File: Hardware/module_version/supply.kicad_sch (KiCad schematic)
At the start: 21 parts, among them J21 Power Input, U32 TLV1117LV33DCYR, U33 TX4139

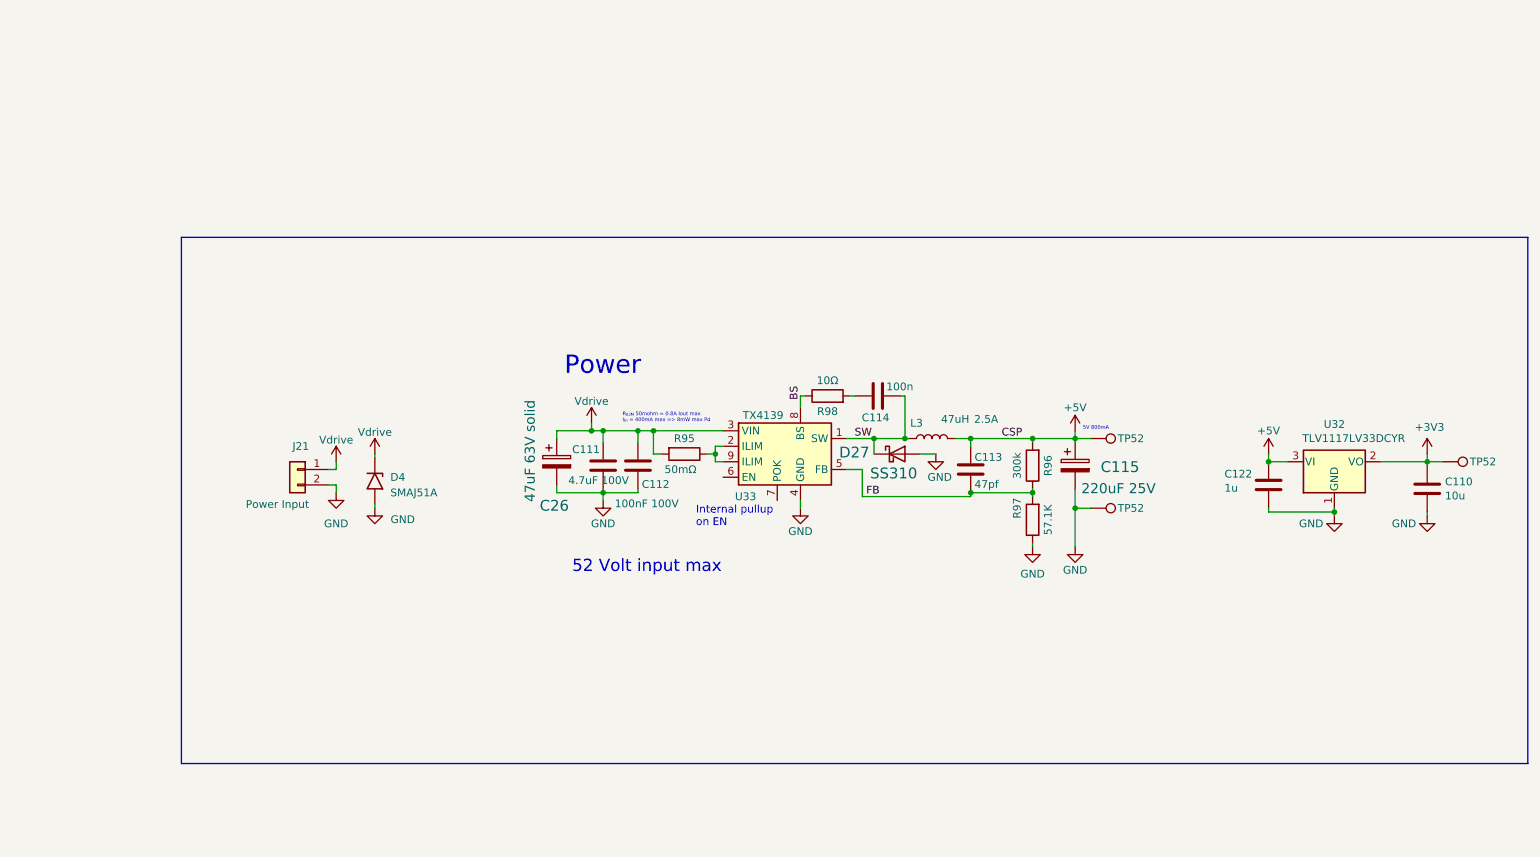
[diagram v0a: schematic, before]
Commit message: work in progress...
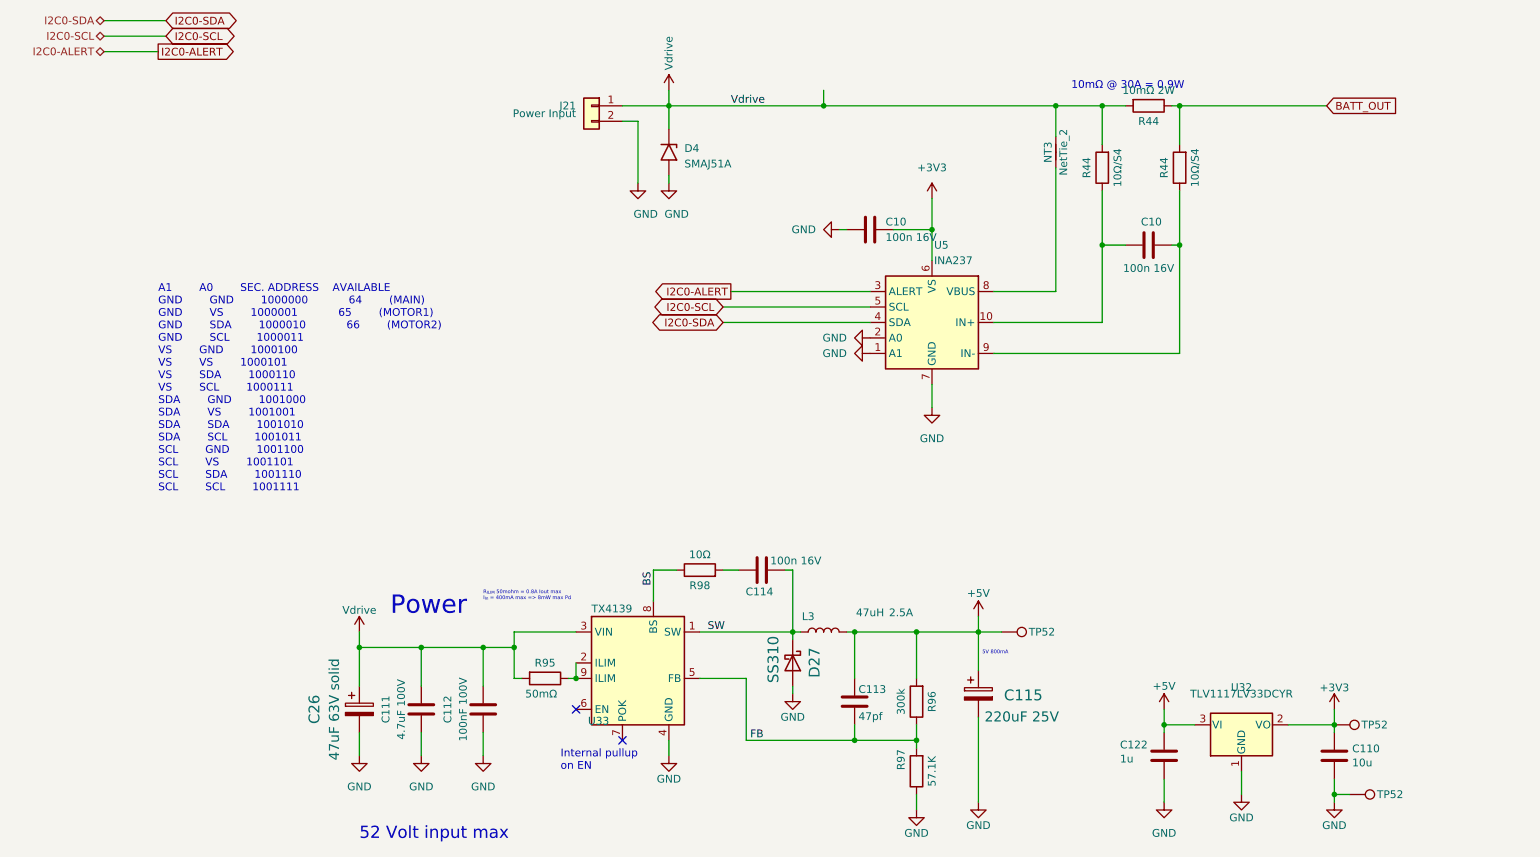
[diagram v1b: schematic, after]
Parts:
- added C10 (x2): 100n 16V, Capacitor_SMD:C_0402_1005Metric, symbol Device:C
- added NT3: NetTie_2, NetTie:NetTie-2_SMD_Pad0.5mm, symbol Device:NetTie_2
- added R44: 10mΩ 2W, Resistor_SMD:R_2512_6332Metric_Pad1.40x3.35mm_HandSolder, symbol Device:R
- added R44 (x2): 10Ω/S4, Resistor_SMD:R_0402_1005Metric, symbol Device:R
- added U5: INA237, Package_SO:VSSOP-10_3x3mm_P0.5mm, symbol katodo_kicad:INA237
- C114: value 100n -> 100n 16V; footprint Capacitor_SMD:C_0603_1608Metric -> Capacitor_SMD:C_0402_1005Metric; LCSC C14663 -> C60474; MFR (none) -> CC0402KRX7R7BB104
- R98: footprint Resistor_SMD:R_0603_1608Metric -> Resistor_SMD:R_0402_1005Metric_Pad0.72x0.64mm_HandSolder; LCSC C22859 -> C138066
- U32: symbol Regulator_Linear:NCP1117-3.3_SOT223 -> katodo_kicad:NCP1117-3.3_SOT223
- U33: symbol MotorBuck:TX4139 -> katodo_kicad:TX4139
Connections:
- net +3V3: now also TP52.1, C10.1, U5.6 (VS); no longer TP52.1
- net GND: now also TP52.1, C10.2, U5.1 (A1), U5.2 (A0), U5.7 (GND); no longer TP52.1
- net Vdrive: now also NT3.2, R44.2, R44.2
- new net: C10.2, R44.1, U5.10 (IN+)
- new net: NT3.1, U5.8 (VBUS)
- new net: C10.1, R44.1, U5.9 (IN-)
- new net BATT_OUT: R44.1, R44.2
- new net I2C0-ALERT: U5.3 (ALERT)
- new net I2C0-SCL: U5.5 (SCL)
- new net I2C0-SDA: U5.4 (SDA)
- no-connect marks 0 -> 2
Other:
- note added: "10mΩ @ 30A = 0.9W"
- note added: "A1 A0 SEC. ADDRESS AVAILABLE GND GND 1000000 64 (MAIN) GND VS 1000001 65 (MOTOR1) GND SDA 1000010 66 (MOTOR2) GND SCL 1000011 VS GND 1000100 VS VS 1000101 VS SDA 1000110 VS SCL 1000111 SDA GND 1001000 SDA VS 1001001 SDA SDA 1001010 SDA SCL 1001011 SCL GND 1001100 SCL VS 1001101 SCL SDA 1001110 SCL SCL 1001111"
- company: Katodo di Mauro Soligo -> Mauro Soligo
- moved on the sheet: C110, C111, C112, C113, C114, C115, C122, C26, D27, D4, J21, L3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
